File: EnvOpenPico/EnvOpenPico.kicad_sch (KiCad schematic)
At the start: 58 parts, among them J2 SKRKAEE020, J3 2.54mm header 01x20, J4 2.54mm header 01x20, J5 Conn_01x03_Male, Q1 Si2329DS, U1 TLV75533PDBVR, U3 RP2040, Y1 3225_4P

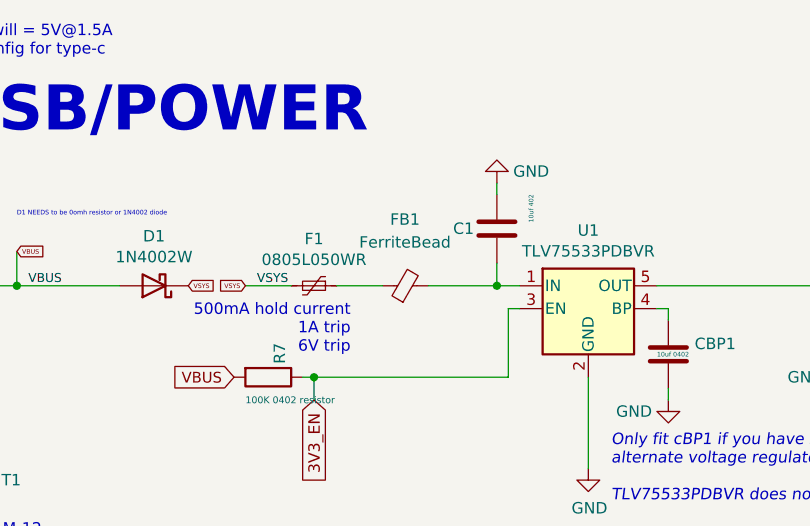
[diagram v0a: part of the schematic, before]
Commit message: tiny cleanup, generated updated gerbers
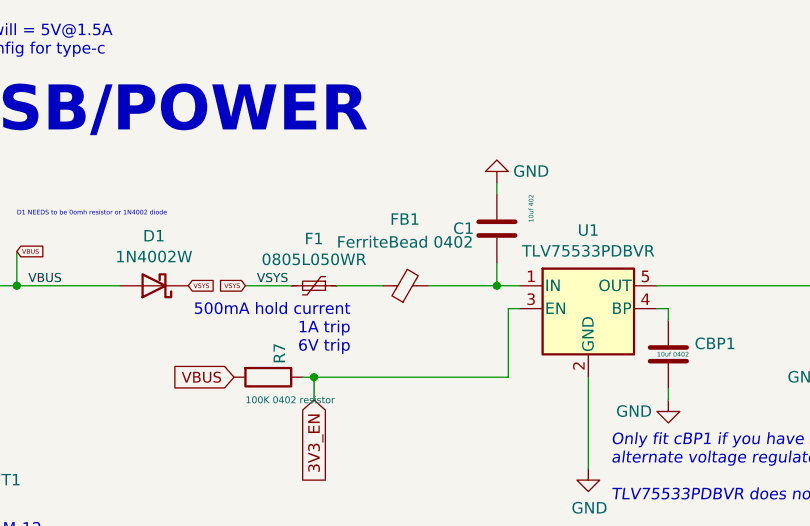
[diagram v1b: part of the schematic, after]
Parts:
- FB1: value FerriteBead -> FerriteBead 0402
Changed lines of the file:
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@@
     (in_bom yes) (on_board yes) (fields_autoplaced)
     (property "Reference" "FB1" (id 0) (at 90.1192 37.084 90))
-    (property "Value" "FerriteBead" (id 1) (at 90.1192 39.624 90))
+    (property "Value" "FerriteBead 0402" (id 1) (at 90.1192 39.624 90))
     (property "Footprint" "Resistor_SMD:R_0402_1005Metric" (id 2) (at 90.17 46.228 90)
       (effects (font (size 1.27 1.27)) hide)
@@
     )
     (path "/cb658bfb-bb44-442b-af68-cdf8168ed728"
-      (reference "FB1") (unit 1) (value "FerriteBead") (footprint "Resistor_SMD:R_0402_1005Metric")
+      (reference "FB1") (unit 1) (value "FerriteBead 0402") (footprint "Resistor_SMD:R_0402_1005Metric")
     )
     (path "/00000000-0000-0000-0000-0000608edada"
